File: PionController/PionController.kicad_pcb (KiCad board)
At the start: 2 copper layers, 1 part, among them U1 STM32H743VITx

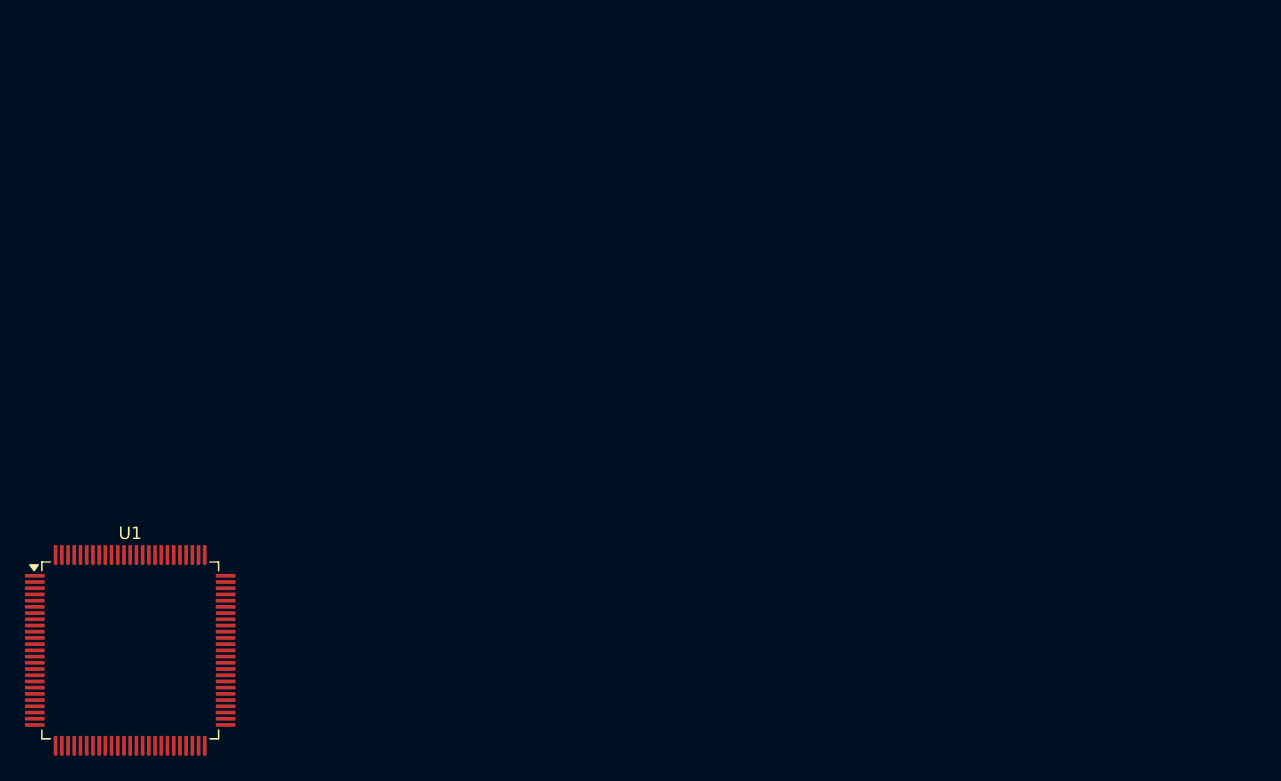
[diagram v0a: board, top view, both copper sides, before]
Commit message: Schematic_ready
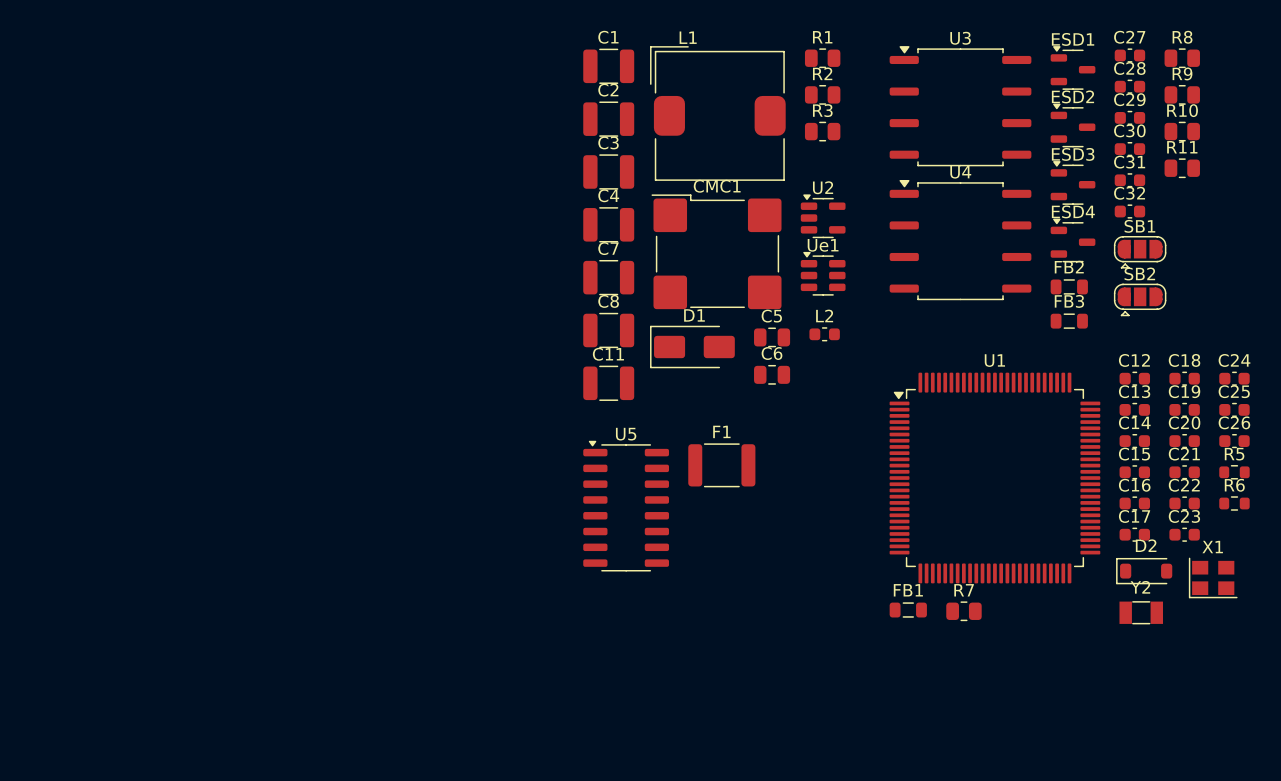
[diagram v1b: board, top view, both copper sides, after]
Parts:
- added C1: 10uF, Capacitor_SMD:C_1210_3225Metric, F.Cu at (138.8, 52.5)
- added C11: 10uF, Capacitor_SMD:C_1210_3225Metric, F.Cu at (138.8, 78.0)
- added C12: 2.2uF, Capacitor_SMD:C_0603_1608Metric, F.Cu at (181.1, 77.6)
- added C13: 2.2uF, Capacitor_SMD:C_0603_1608Metric, F.Cu at (181.1, 80.2)
- added C14: 100nF, Capacitor_SMD:C_0603_1608Metric, F.Cu at (181.1, 82.7)
- added C15: 100nF, Capacitor_SMD:C_0603_1608Metric, F.Cu at (181.1, 85.2)
- added C16: 100nF, Capacitor_SMD:C_0603_1608Metric, F.Cu at (181.1, 87.7)
- added C17: 100nF, Capacitor_SMD:C_0603_1608Metric, F.Cu at (181.1, 90.2)
- added C18: 100nF, Capacitor_SMD:C_0603_1608Metric, F.Cu at (185.2, 77.6)
- added C19: 100nF, Capacitor_SMD:C_0603_1608Metric, F.Cu at (185.2, 80.2)
- added C2: 10uF, Capacitor_SMD:C_1210_3225Metric, F.Cu at (138.8, 56.8)
- added C20: 2.2uF, Capacitor_SMD:C_0603_1608Metric, F.Cu at (185.2, 82.7)
- added C21: 2.2uF, Capacitor_SMD:C_0603_1608Metric, F.Cu at (185.2, 85.2)
- added C22: 100nF, Capacitor_SMD:C_0603_1608Metric, F.Cu at (185.2, 87.7)
- added C23: 100nF, Capacitor_SMD:C_0603_1608Metric, F.Cu at (185.2, 90.2)
- added C24: 22pF, Capacitor_SMD:C_0603_1608Metric, F.Cu at (189.2, 77.6)
- added C25: 22pF, Capacitor_SMD:C_0603_1608Metric, F.Cu at (189.2, 80.2)
- added C26: 2.2uF, Capacitor_SMD:C_0603_1608Metric, F.Cu at (189.2, 82.7)
- added C27: 100nF, Capacitor_SMD:C_0603_1608Metric, F.Cu at (180.8, 51.6)
- added C28: 100nF, Capacitor_SMD:C_0603_1608Metric, F.Cu at (180.8, 54.2)
- added C29: 100nF, Capacitor_SMD:C_0603_1608Metric, F.Cu at (180.8, 56.7)
- added C3: 10uF, Capacitor_SMD:C_1210_3225Metric, F.Cu at (138.8, 61.0)
- added C30: 100nF, Capacitor_SMD:C_0603_1608Metric, F.Cu at (180.8, 59.2)
- added C31: 100nF, Capacitor_SMD:C_0603_1608Metric, F.Cu at (180.8, 61.7)
- added C32: 100nF, Capacitor_SMD:C_0603_1608Metric, F.Cu at (180.8, 64.2)
- added C4: 10uF, Capacitor_SMD:C_1210_3225Metric, F.Cu at (138.8, 65.3)
- added C5: 100nF, Capacitor_SMD:C_0805_2012Metric, F.Cu at (152.0, 74.3)
- added C6: 100nF, Capacitor_SMD:C_0805_2012Metric, F.Cu at (152.0, 77.3)
- added C7: 10uF, Capacitor_SMD:C_1210_3225Metric, F.Cu at (138.8, 69.5)
- added C8: 10uF, Capacitor_SMD:C_1210_3225Metric, F.Cu at (138.8, 73.8)
- added CMC1: PSMCAQ1050-801P, Inductor_SMD:L_CommonModeChoke_Wuerth_WE-SL5, F.Cu at (147.6, 67.6)
- added D1: SMAJ18A, Diode_SMD:D_SMA, F.Cu at (145.7, 75.1)
- added D2: 1N5819W1, Diode_SMD:D_SOD-123, F.Cu at (182.1, 93.1)
- added ESD1: CDSOT23-SM712, Package_TO_SOT_SMD:SOT-23-3, F.Cu at (176.2, 52.8)
- added ESD2: CDSOT23-SM712, Package_TO_SOT_SMD:SOT-23-3, F.Cu at (176.2, 57.4)
- added ESD3: CDSOT23-SM712, Package_TO_SOT_SMD:SOT-23-3, F.Cu at (176.2, 62.0)
- added ESD4: CDSOT23-SM712, Package_TO_SOT_SMD:SOT-23-3, F.Cu at (176.2, 66.7)
- added F1: 2.6A PPTC, Fuse:Fuse_1812_4532Metric, F.Cu at (147.9, 84.6)
- added FB1: 200R/100MHz 500mA, Inductor_SMD:L_0805_2012Metric, F.Cu at (162.9, 96.3)
- added FB2: 200R/100MHz 500mA, Inductor_SMD:L_0805_2012Metric, F.Cu at (175.9, 70.3)
- added FB3: 200R/100MHz 500mA, Inductor_SMD:L_0805_2012Metric, F.Cu at (175.9, 73.0)
- added L1: 33uH, Inductor_SMD:L_TDK_SLF10145, F.Cu at (147.8, 56.5)
- added L2: 4.7uH, Inductor_SMD:L_0603_1608Metric, F.Cu at (156.2, 74.1)
- added R1: 54.9K, Resistor_SMD:R_0805_2012Metric, F.Cu at (156.0, 51.9)
- added R10: 60.4, Resistor_SMD:R_0805_2012Metric, F.Cu at (185.0, 57.8)
- added R11: 60.4, Resistor_SMD:R_0805_2012Metric, F.Cu at (185.0, 60.7)
- added R2: 10K, Resistor_SMD:R_0805_2012Metric, F.Cu at (156.0, 54.8)
- added R3: 10K, Resistor_SMD:R_0805_2012Metric, F.Cu at (156.0, 57.8)
- added R5: 0, Resistor_SMD:R_0603_1608Metric, F.Cu at (189.2, 85.2)
- added R6: 0, Resistor_SMD:R_0603_1608Metric, F.Cu at (189.2, 87.7)
- added R7: 10K, Resistor_SMD:R_0805_2012Metric, F.Cu at (167.4, 96.4)
- added R8: 60.4, Resistor_SMD:R_0805_2012Metric, F.Cu at (185.0, 51.9)
- added R9: 60.4, Resistor_SMD:R_0805_2012Metric, F.Cu at (185.0, 54.8)
- added SB1: TERM, Jumper:SolderJumper-3_P1.3mm_Open_RoundedPad1.0x1.5mm, F.Cu at (181.6, 67.2)
- added SB2: TERM, Jumper:SolderJumper-3_P1.3mm_Open_RoundedPad1.0x1.5mm, F.Cu at (181.6, 71.1)
- added U2: TLV75733PDBV, Package_TO_SOT_SMD:SOT-23-5, F.Cu at (156.1, 64.7)
- added U3: ISO1050DUB, Package_SO:SOP-8_6.62x9.15mm_P2.54mm, F.Cu at (167.1, 55.8)
- added U4: ISO1050DUB, Package_SO:SOP-8_6.62x9.15mm_P2.54mm, F.Cu at (167.1, 66.6)
- added U5: CA-IS3740HN, Package_SO:SOIC-16_3.9x9.9mm_P1.27mm, F.Cu at (140.2, 88.0)
- added Ue1: TPS562200, Package_TO_SOT_SMD:SOT-23-6, F.Cu at (156.1, 69.3)
- added X1: ASE-16.00MHz, Oscillator:Oscillator_SMD_Abracon_ASE-4Pin_3.2x2.5mm, F.Cu at (187.4, 93.7)
- added Y2: 32.768kHZ, Crystal:Crystal_SMD_3215-2Pin_3.2x1.5mm, F.Cu at (181.7, 96.5)
- moved U1 70.9 mm to (169.9, 85.6)
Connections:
- U1 pad 10: Net-(U1-VSS-Pad10) -> GND
- U1 pad 100: unconnected-(U1-VDD-Pad100) -> +3.3V
- U1 pad 11: unconnected-(U1-VDD-Pad11) -> +3.3V
- U1 pad 12: unconnected-(U1-PH0-Pad12) -> HSE_IN
- U1 pad 19: unconnected-(U1-VSSA-Pad19) -> GND
- U1 pad 20: unconnected-(U1-VREF+-Pad20) -> VREF
- U1 pad 21: unconnected-(U1-VDDA-Pad21) -> VDDA
- U1 pad 26: Net-(U1-VSS-Pad10) -> GND
- U1 pad 27: unconnected-(U1-VDD-Pad27) -> +3.3V
- U1 pad 48: unconnected-(U1-VCAP-Pad48) -> Net-(C12-Pad2)
- U1 pad 49: Net-(U1-VSS-Pad10) -> GND
- U1 pad 50: unconnected-(U1-VDD-Pad50) -> +3.3V
- U1 pad 6: unconnected-(U1-VBAT-Pad6) -> +3.3V
- U1 pad 73: unconnected-(U1-VCAP-Pad73) -> Net-(C13-Pad2)
- U1 pad 74: Net-(U1-VSS-Pad10) -> GND
- U1 pad 75: unconnected-(U1-VDD-Pad75) -> +3.3V
- U1 pad 8: unconnected-(U1-PC14-Pad8) -> LSE_OSC_IN
- U1 pad 9: unconnected-(U1-PC15-Pad9) -> LSE_OSC_OUT
- U1 pad 91: unconnected-(U1-PB5-Pad91) -> CAN_COMM_RX
- U1 pad 92: unconnected-(U1-PB6-Pad92) -> CAN_COMM_TX
- U1 pad 95: unconnected-(U1-PB8-Pad95) -> CAN_CRIT_RX
- U1 pad 96: unconnected-(U1-PB9-Pad96) -> CAN_CRIT_TX
- U1 pad 99: Net-(U1-VSS-Pad10) -> GND
